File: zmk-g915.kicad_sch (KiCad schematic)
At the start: 53 parts, among them J1 Prog_conn, J2 Tag connect TC2030-CTX, J3 53047-0460, Q3 Q_NMOS, SW1 Reset Switch, U1 nRF52840-QIAA-R/nRF52833-QIAA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, U2 SN74AHCT1G125, Y1 32.768kHz, Y2 32MHz

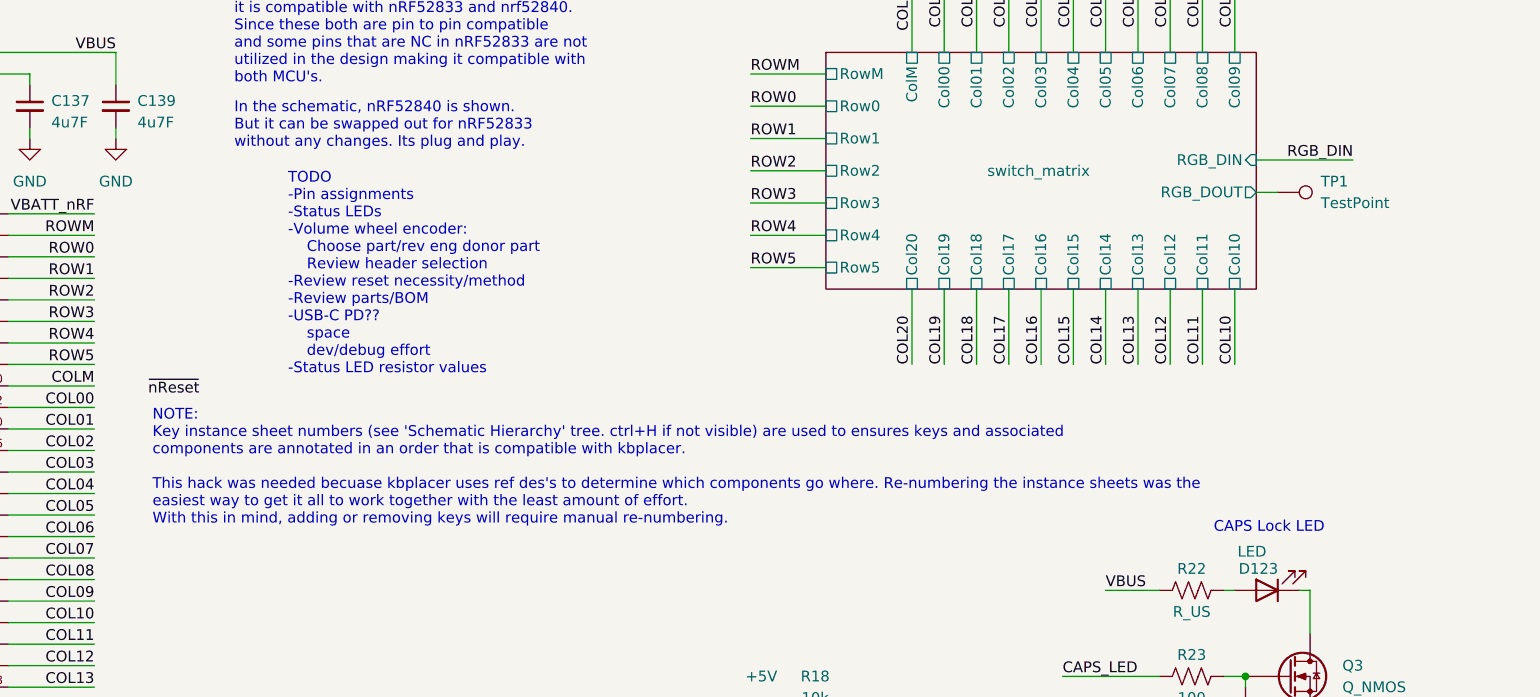
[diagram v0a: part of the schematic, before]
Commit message: Power supply and PCB stuff
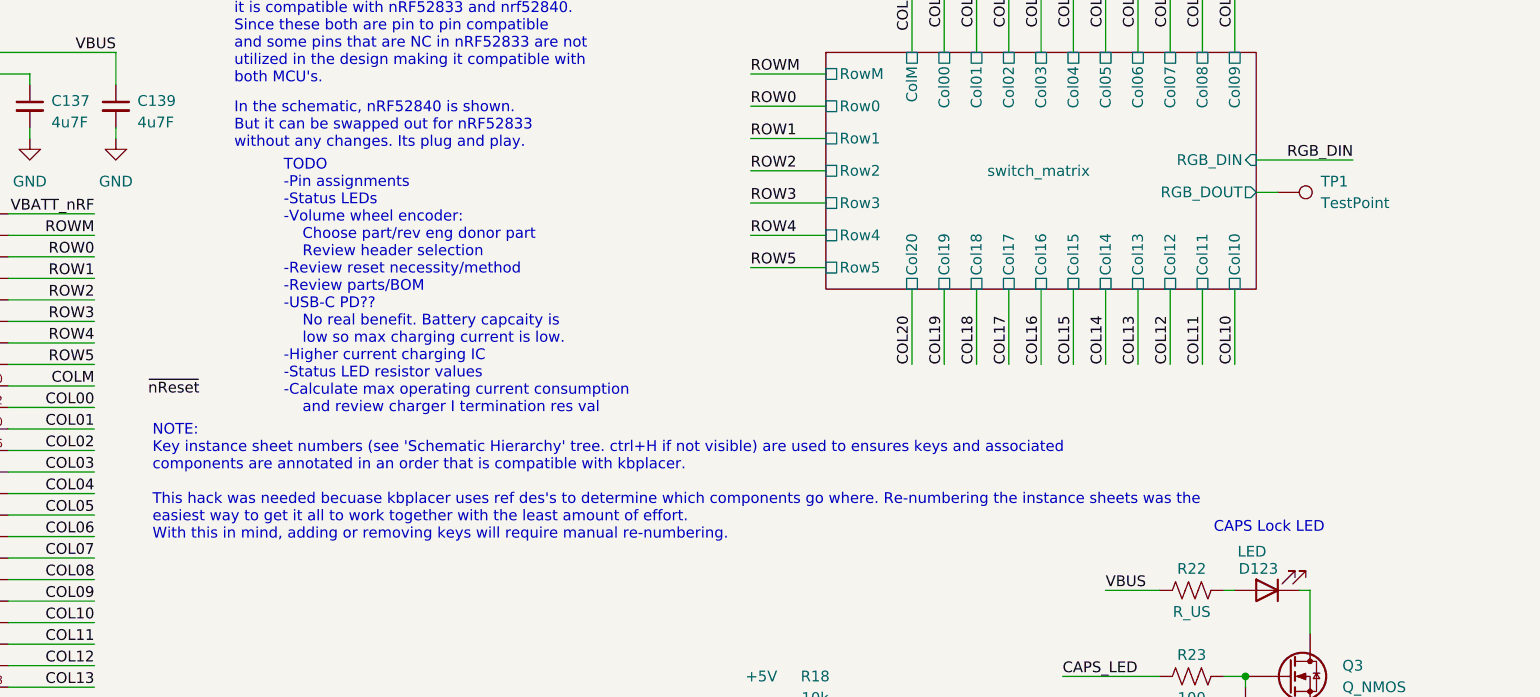
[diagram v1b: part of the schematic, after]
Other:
- note added: "TODO -Pin assignments -Status LEDs -Volume wheel encoder: Choose part/rev eng donor part Review header selection -Review reset necessity/method -Review parts/BOM -USB-C PD?? No real benefit. Battery capcaity is low so max charging current is low. -Higher current charging IC -Status LED resistor values -Calculate max operating current consumption and review charger I termination res val"
- note removed: "TODO -Pin assignments -Status LEDs -Volume wheel encoder: Choose part/rev eng donor part Review header selection -Review reset necessity/method -Review parts/BOM -USB-C PD?? space dev/debug effort -Status LED resistor values"
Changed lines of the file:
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@@
 	(text "NOTE:\nKey instance sheet numbers (see 'Schematic Hierarchy' tree. ctrl+H if not visible) are used to ensures keys and associated\ncomponents are annotated in an order that is compatible with kbplacer.\n\nThis hack was needed becuase kbplacer uses ref des's to determine which components go where. Re-numbering the instance sheets was the\neasiest way to get it all to work together with the least amount of effort.\nWith this in mind, adding or removing keys will require manual re-numbering."
 		(exclude_from_sim no)
-		(at 136.398 102.362 0)
+		(at 136.398 104.14 0)
 		(effects
 			(font
@@
 		)
 	)
-	(text "TODO\n-Pin assignments\n-Status LEDs\n-Volume wheel encoder:\n	Choose part/rev eng donor part\n	Review header selection\n-Review reset necessity/method\n-Review parts/BOM\n-USB-C PD??\n	space\n	dev/debug effort\n-Status LED resistor values"
+	(text "TODO\n-Pin assignments\n-Status LEDs\n-Volume wheel encoder:\n	Choose part/rev eng donor part\n	Review header selection\n-Review reset necessity/method\n-Review parts/BOM\n-USB-C PD??\n	No real benefit. Battery capcaity is\n	low so max charging current is low.\n-Higher current charging IC\n-Status LED resistor values\n-Calculate max operating current consumption\n	and review charger I termination res val"
 		(exclude_from_sim no)
-		(at 152.4 79.502 0)
+		(at 151.892 81.026 0)
 		(effects
 			(font
